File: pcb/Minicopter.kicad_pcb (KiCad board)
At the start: 2 copper layers, 80 x 80 mm, 57 parts, among them J1 USB_C_Receptacle_USB2.0_16P, J2 Conn_01x02, J3 Conn_01x02_Socket, J4 Conn_01x02_Socket, J5 Conn_01x02_Socket, J6 Conn_01x02_Socket, Q1 AO3401A, SW1 SS-12D00, T1 IRLML6344TRPBF, T2 IRLML6344TRPBF, T3 IRLML6344TRPBF, T4 IRLML6344TRPBF, U1 SPX3819M5-L-3-3, U2 TP4056-42-ESOP8, U3 ESP32-C3-WROOM-02, U4 GY-87_Module, U5 USBLC6-2P6

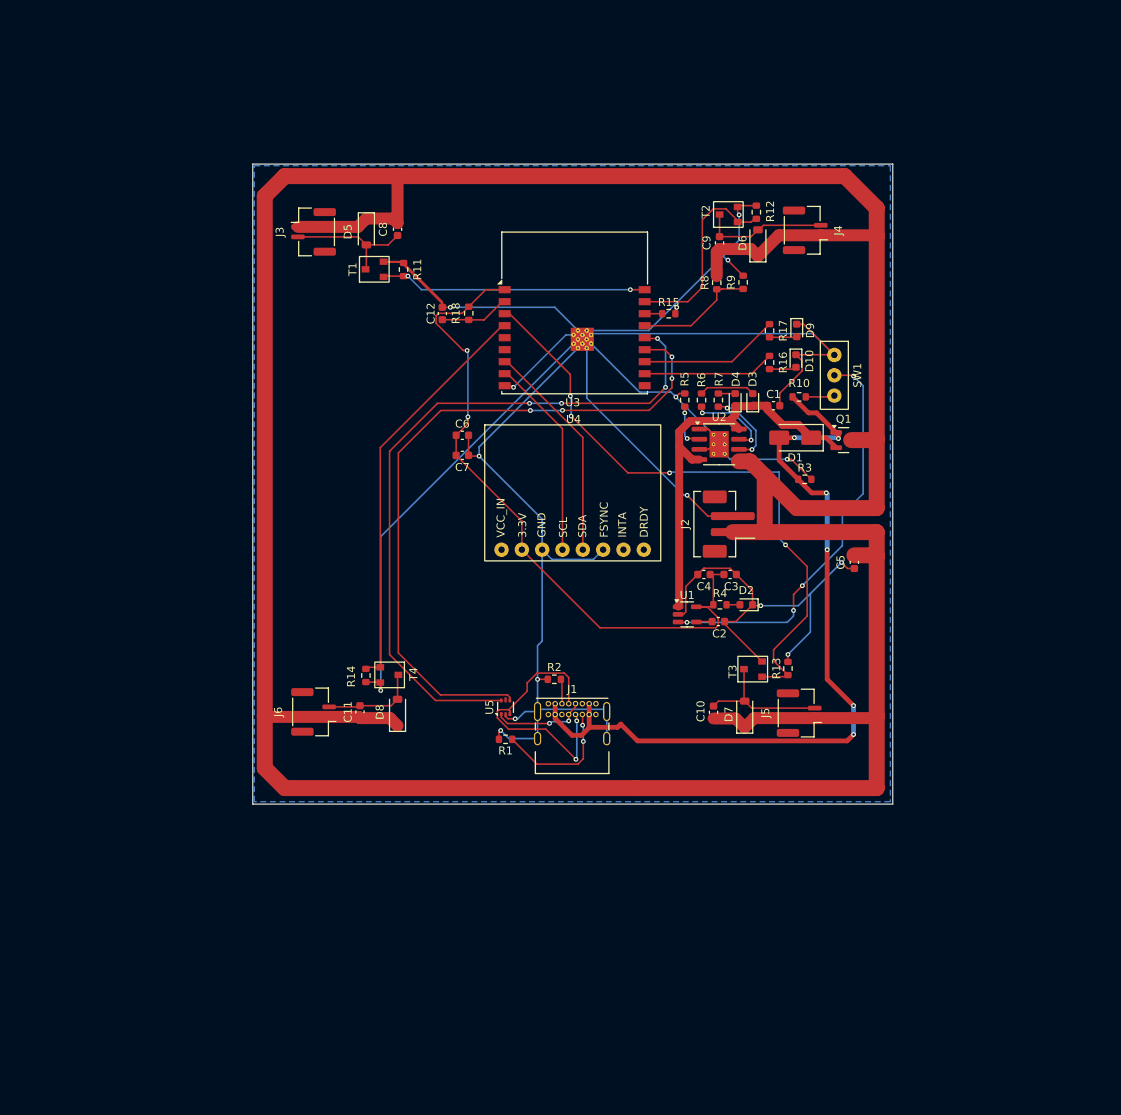
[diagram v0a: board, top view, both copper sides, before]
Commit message: oops now done hopefully
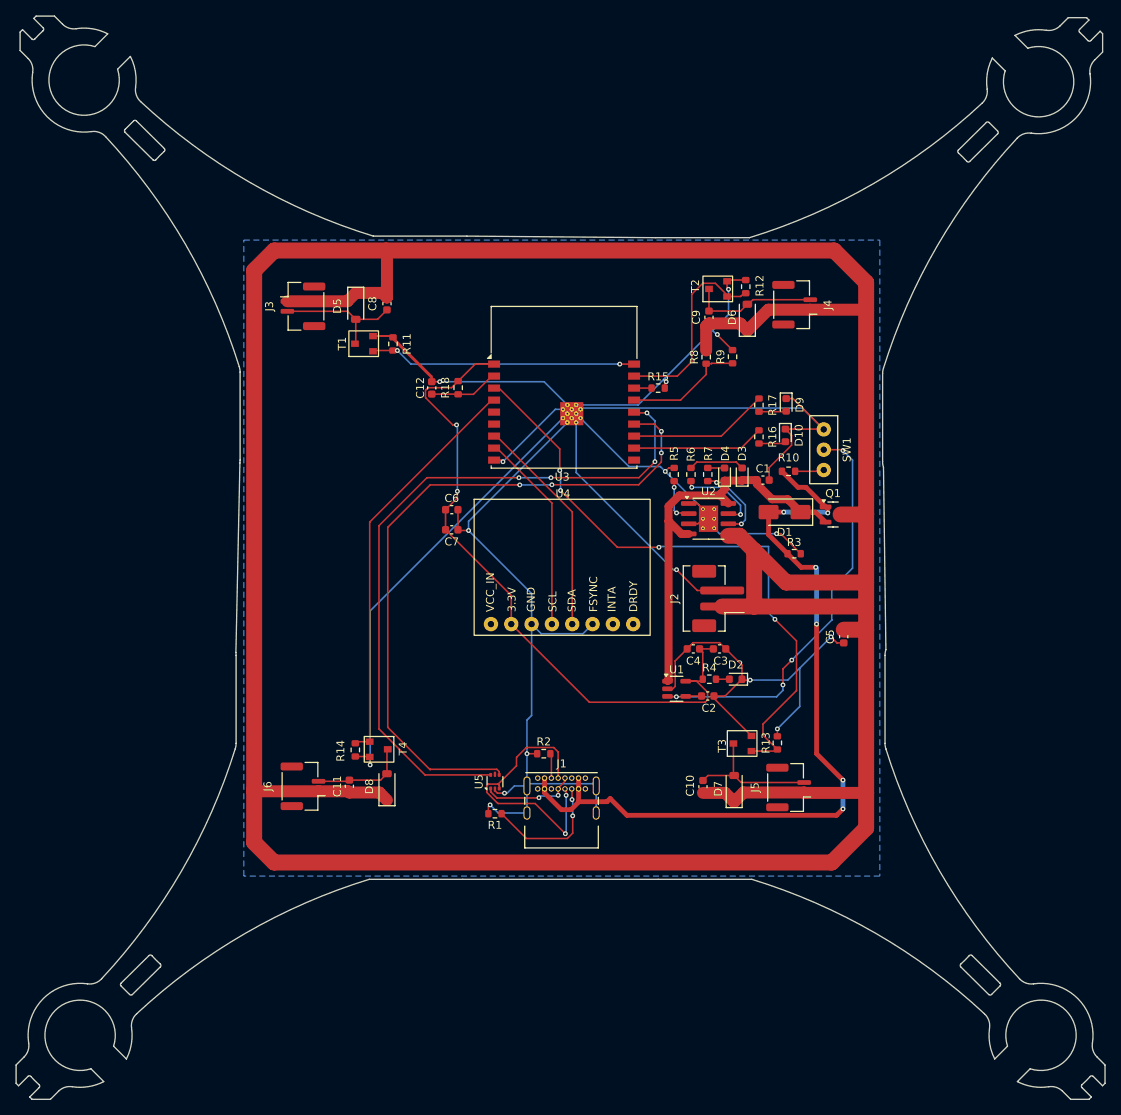
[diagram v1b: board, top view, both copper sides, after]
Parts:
- moved C11 9.39 mm to (123.1, 123.8)
- moved C3 9.39 mm to (169.4, 106.6)
- moved C4 9.39 mm to (166.1, 106.6)
- moved D10 9.39 mm to (177.6, 79.9)
- moved D3 9.39 mm to (172.2, 84.8)
- moved D4 9.39 mm to (170.0, 84.8)
- moved R10 9.39 mm to (178.0, 84.4)
- moved R13 9.39 mm to (176.6, 118.4)
- moved R14 9.39 mm to (123.8, 119.2)
- moved D8 9.39 mm to (127.8, 123.9)
- moved J6 9.39 mm to (117.3, 123.8)
- moved T4 9.39 mm to (125.1, 119.2)
- moved C12 9.39 mm to (133.4, 74.0)
- moved C2 9.39 mm to (167.9, 112.5)
- moved C7 9.39 mm to (135.9, 91.7)
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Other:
- board size 80 x 80 mm -> 136.1 x 135.4 mm
